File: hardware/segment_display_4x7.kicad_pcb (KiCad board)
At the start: 2 copper layers, 65 x 25 mm, 21 parts, among them P1 CON-SENSOR, U1 M24C64, U2 TM1637, U3 SEGMENT_4X7, U4 DRILL, U5 DRILL, U6 DRILL, U7 DRILL

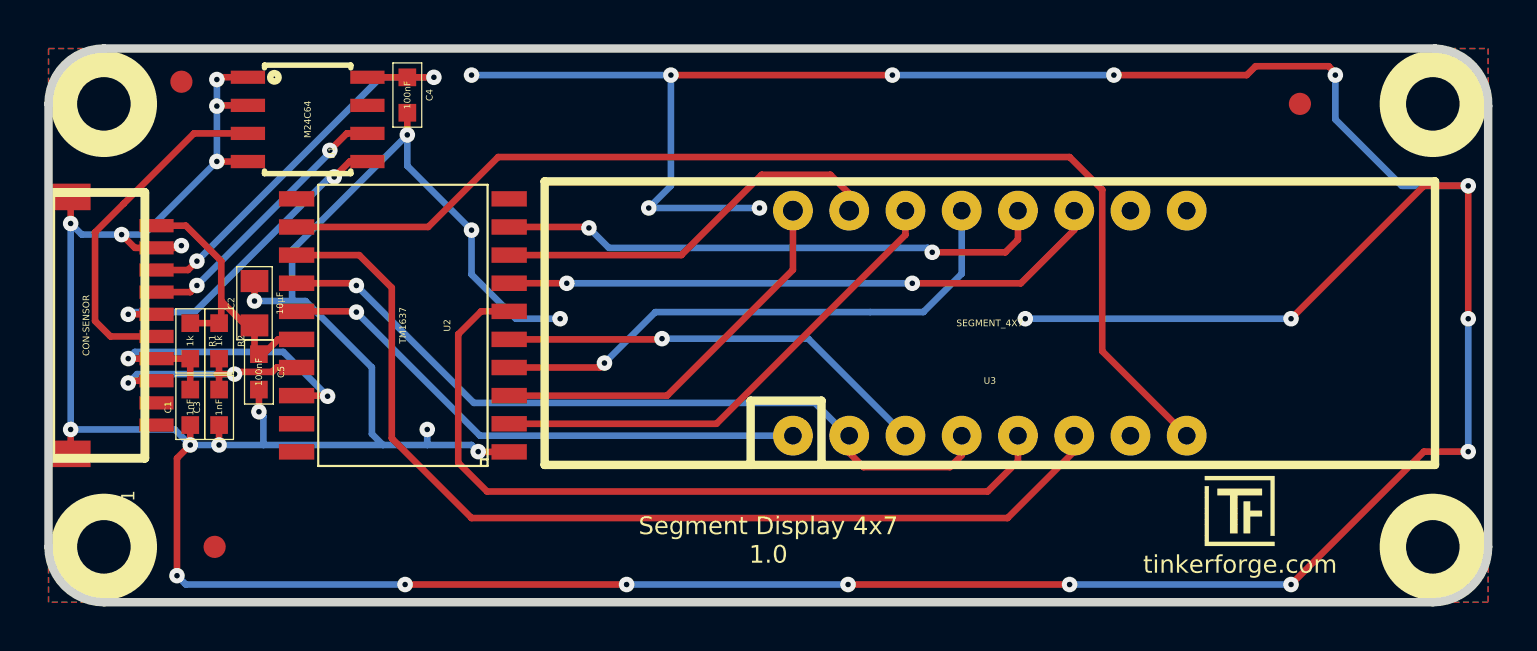
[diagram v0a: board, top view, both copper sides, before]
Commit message: Add 3d information (final)
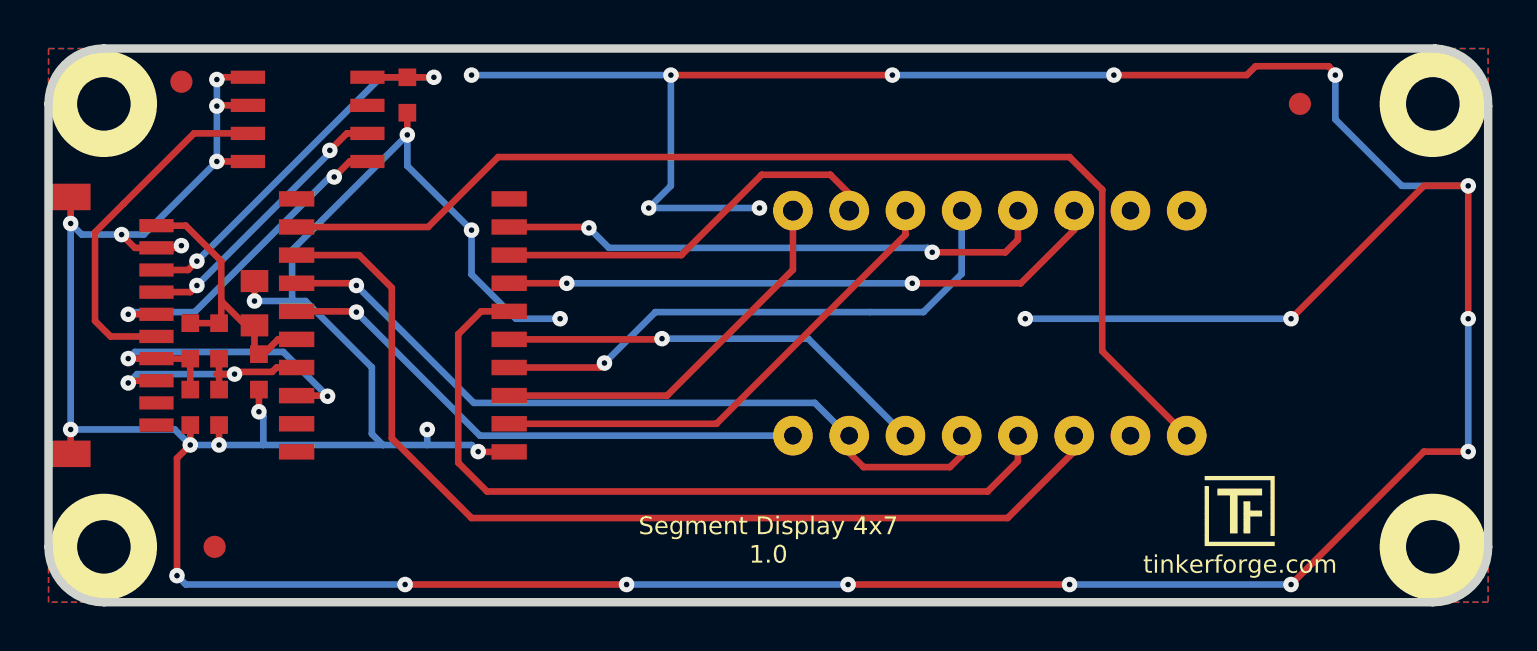
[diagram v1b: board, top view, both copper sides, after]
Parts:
- C1, C3, C4: footprint 0603 -> kicad-libraries:C0603
- C2: footprint 0805 -> kicad-libraries:C0805
- C5, R1, R2: footprint 0603 -> kicad-libraries:R0603
- Fiducial_Mark (x3): footprint Fiducial_Mark -> kicad-libraries:Fiducial_Mark
- G***: footprint Logo_31x31 -> kicad-libraries:Logo_31x31
- P1: footprint CON-SENSOR -> kicad-libraries:CON-SENSOR
- U1: footprint SOIC8 -> kicad-libraries:SOIC8
- U2: footprint SOP20 -> kicad-libraries:SOP20
- U3: footprint SEGMENT_4X7 -> kicad-libraries:SEGMENT_4X7
- U4, U5, U6, U7: footprint DRILL_NP -> kicad-libraries:DRILL_NP
- VAL: footprint CE_5mm -> kicad-libraries:CE_5mm
- VAL: footprint WEEE_7mm -> kicad-libraries:WEEE_7mm
- turned VAL to 180 degrees
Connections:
- P1 pad 10: (no net) -> Net-(P1-Pad10)
- P1 pad 9: (no net) -> Net-(P1-Pad9)
- U1 pad 7: (no net) -> Net-(U1-Pad7)
- U2 pad 10: (no net) -> Net-(U2-Pad10)
- U2 pad 11: (no net) -> Net-(U2-Pad11)
- U2 pad 19: (no net) -> Net-(U2-Pad19)
- U2 pad 20: (no net) -> Net-(U2-Pad20)
- U3 pad 10: (no net) -> Net-(U3-Pad10)
- U3 pad 7: (no net) -> Net-(U3-Pad7)
- U3 pad 9: (no net) -> Net-(U3-Pad9)
